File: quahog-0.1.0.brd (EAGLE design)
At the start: 71.3 x 17.9 mm, 33 parts, among them IC3 MCP1703CB, IC5 24AA128SN, J1 AYZ0202, X1 16 MHz

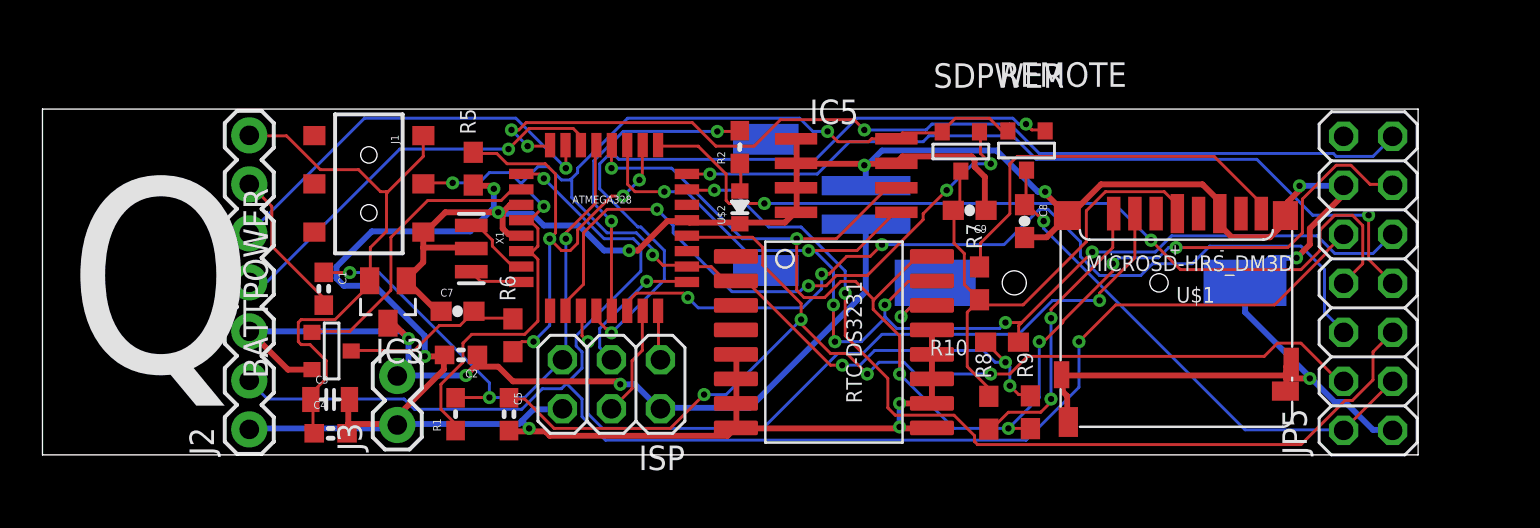
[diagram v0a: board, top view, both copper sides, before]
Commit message: update
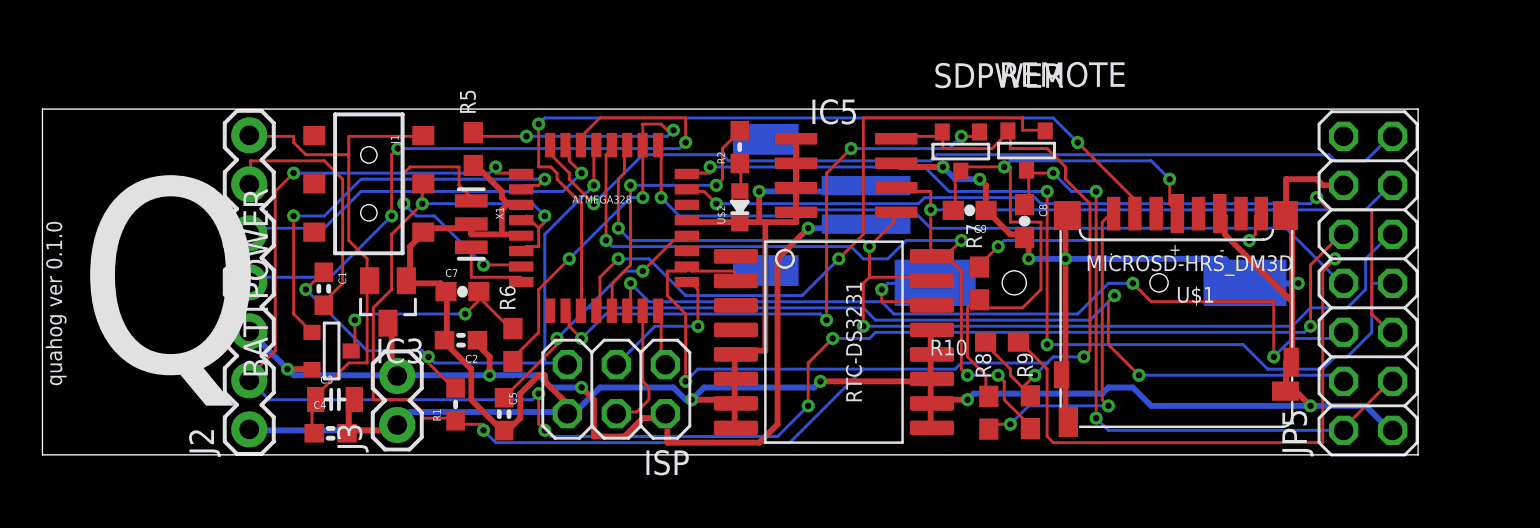
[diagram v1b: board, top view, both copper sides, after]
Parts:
- moved X1 1.27 mm to (22.2, 12.0)
- moved C7 1.05 mm to (21.8, 8.46)
- moved R5 1.02 mm to (22.3, 15.8)
- moved C2 0.76 mm to (21.7, 5.94)
- moved R1 0.51 mm to (21.4, 2.62)
- moved R6 0.51 mm to (24.4, 5.69)
- moved ISP 0.36 mm to (29.7, 3.40)
- moved C5 0.25 mm to (23.9, 2.11)
- moved C3 0.25 mm to (15.2, 2.87)
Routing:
- net SDA: track 60.8 -> 89.5 mm, vias 7 -> 4
- net VCC: track 86.2 -> 110.6 mm, vias 7 -> 6
- net D0_RX: track 21.1 -> 35.1 mm, vias 1 -> 3
- net N$1: track 3.66 -> 14.0 mm, vias 0 -> 2
- net D3: track 82.2 -> 90.6 mm, vias 2 -> 7
- net GND: track 201.4 -> 193.7 mm, vias 12 -> 10
- net N$7: track 27.1 -> 34.5 mm, vias 1 -> 3
- net A1: track 41.9 -> 49.2 mm, vias 2 -> 3
- net N$4: track 27.6 -> 33.9 mm, vias 0 -> 2
- net D4: track 15.5 -> 21.7 mm, vias 0 -> 2
- net N$20: track 7.88 -> 13.3 mm
- net A2: track 45.4 -> 40.3 mm, vias 2 -> 1
- net PWR: track 48.4 -> 53.5 mm, vias 3 -> 4
- net A0: track 48.3 -> 43.3 mm
- net N$16: track 20.7 -> 16.3 mm, vias 0 -> 2
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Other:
- board text added: "quahog ver 0.1.0"

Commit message: update
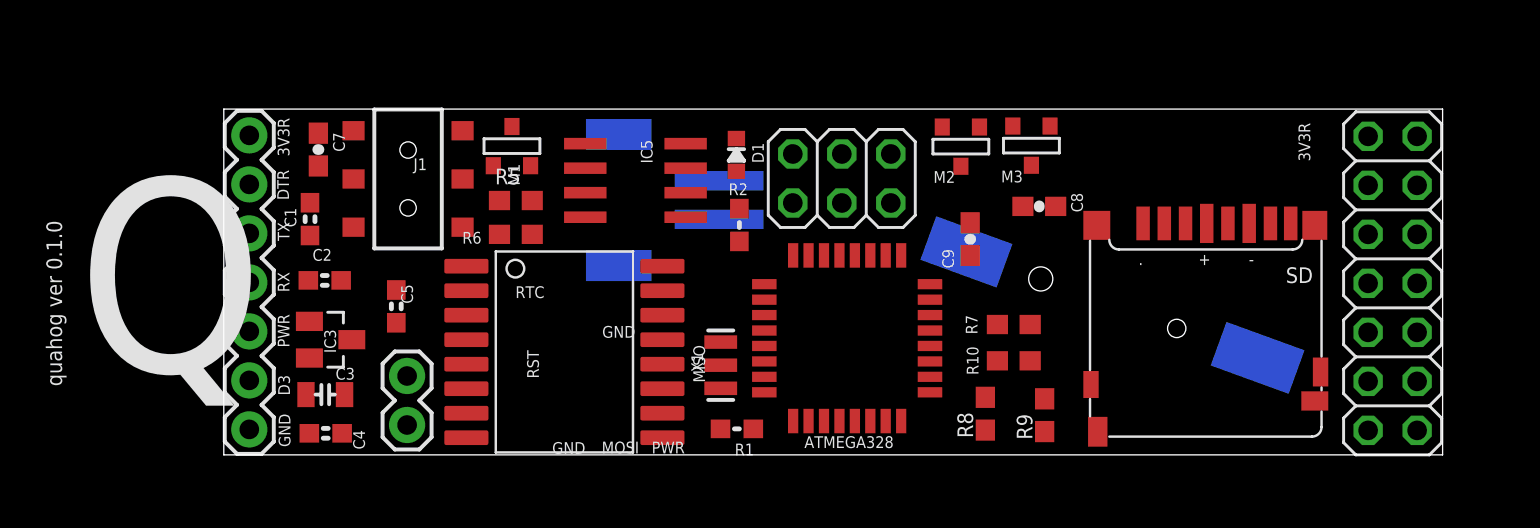
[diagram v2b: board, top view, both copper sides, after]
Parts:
- removed BATTPOWER, REMOTE, SDPWER: FDN340P, zetex:SOT-23
- removed RTC-DS3231: DS3231, _lh-library:DS3231
- removed U$1: MICROSD-HRS_DM3D, hrs_DM3D-SF:DM3D
- removed U$2: LED0603, LowPowerLab:0603-LED
- added D1: LED0603, LowPowerLab:0603-LED
- added M1, M2, M3: FDN340P, zetex:SOT-23
- added RTC: DS3231, _lh-library:DS3231
- added SD: MICROSD-HRS_DM3D, hrs_DM3D-SF:DM3D
- moved ISP 16.0 mm to (41.4, 14.3)
- moved X1 14.9 mm to (35.2, 4.65)
- moved R1 14.6 mm to (36.0, 1.35), turned to 180 degrees
- moved ATMEGA328 13.8 mm to (41.7, 6.05), turned to 180 degrees
- moved IC5 10.9 mm to (30.7, 14.2), turned to 90 degrees
- moved C7 10.5 mm to (14.3, 15.8), turned to 270 degrees
- moved C5 7.90 mm to (18.3, 7.70)
- moved C2 7.71 mm to (14.6, 9.04), turned to 0 degrees
- moved CN2 7.62 mm to (31.4, 13.2)
- moved R6 5.74 mm to (24.5, 11.4), turned to 180 degrees
- moved R2 4.04 mm to (36.1, 11.9), turned to 270 degrees
- moved C1 3.68 mm to (13.9, 12.2), turned to 90 degrees
- moved IC3 3.56 mm to (14.9, 5.97), turned to 270 degrees
- moved R5 3.46 mm to (24.5, 13.2), turned to 180 degrees
- moved R7 2.78 mm to (50.3, 6.76), turned to 180 degrees
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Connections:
- removed net D11_MOSI: ATMEGA328.15, ISP.4
- removed net D12_MISO: ATMEGA328.16, ISP.1
- removed net D13_SCK: ATMEGA328.17, ISP.3
- removed net D5/RTC: RTC-DS3231.3
- removed net VBAT: JP5.14
- net A2: now also JP5.10; no longer JP5.8
- net A3: now also JP5.8
- net AREF: now also JP5.2; no longer JP5.4
- net D10: now also JP5.4; no longer JP5.6
- net D3: now also JP5.6; no longer JP5.10
- net D4: now also M1.3; no longer BATTPOWER.3
- net D5: now also RTC.3
- net D6: now also M2.3; no longer SDPWER.3
- net D7: now also SD.CD/DAT3; no longer U$1.CD/DAT3
- net D8: now also M3.3; no longer REMOTE.3
- net GND: now also D1.MINUS, RTC.10, RTC.11, RTC.12, RTC.13, RTC.5, RTC.6, RTC.7, RTC.8, RTC.9, SD.GND1, SD.GND2, SD.GND3, SD.GND4, SD.SW_A, SD.SW_B, SD.VSS; no longer RTC-DS3231.10, RTC-DS3231.11, RTC-DS3231.12, RTC-DS3231.13, RTC-DS3231.5, RTC-DS3231.6, RTC-DS3231.7, RTC-DS3231.8, RTC-DS3231.9, U$1.GND1, U$1.GND2, U$1.GND3, U$1.GND4, U$1.SW_A, U$1.SW_B, U$1.VSS, U$2.MINUS
- net MISO: now also ATMEGA328.16, ISP.1, SD.DAT0; no longer U$1.DAT0
- net MOSI: now also ATMEGA328.15, ISP.4, SD.CMD; no longer U$1.CMD
- net N$15: now also M1.1; no longer BATTPOWER.1
- net N$16: now also SD.DAT1; no longer U$1.DAT1
- net N$18: now also SD.DAT2; no longer U$1.DAT2
- net N$2: now also D1.PLUS; no longer U$2.PLUS
- net N$4: now also M2.1, SD.VDD; no longer SDPWER.1, U$1.VDD
- net N$7: now also M3.1; no longer JP5.2, REMOTE.1
- net PWR: now also JP5.14, M1.2; no longer BATTPOWER.2
- net RTC_BATT: now also RTC.14; no longer RTC-DS3231.14
- net SCK: now also ATMEGA328.17, ISP.3, SD.CLK; no longer U$1.CLK
- net SCL: now also RTC.16; no longer RTC-DS3231.16
- net SDA: now also RTC.15; no longer RTC-DS3231.15
- net VCC: now also M2.2, M3.2, RTC.2; no longer REMOTE.2, RTC-DS3231.2, SDPWER.2
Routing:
- net GND: track 193.7 -> 0.00 mm, vias 10 -> 0
- net VCC: track 110.6 -> 0.00 mm, vias 6 -> 0
- net D3: track 90.6 -> 0.00 mm, vias 7 -> 0
- net SDA: track 89.5 -> 0.00 mm, vias 4 -> 0
- net SCL: track 68.5 -> 0.00 mm, vias 5 -> 0
- net AREF: track 57.0 -> 0.00 mm, vias 4 -> 0
- net PWR: track 53.5 -> 0.00 mm, vias 4 -> 0
- net A1: track 49.2 -> 0.00 mm, vias 3 -> 0
- net D2: track 47.3 -> 0.00 mm, vias 1 -> 0
- net D7: track 44.5 -> 0.00 mm, vias 2 -> 0
- net D10: track 43.5 -> 0.00 mm, vias 3 -> 0
- net A0: track 43.3 -> 0.00 mm, vias 2 -> 0
- net A2: track 40.3 -> 0.00 mm, vias 1 -> 0
- net D0_RX: track 35.1 -> 0.00 mm, vias 3 -> 0
- net N$7: track 34.5 -> 0.00 mm, vias 3 -> 0
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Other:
- board size 71.3 x 17.9 mm -> 63.2 x 17.9 mm
- board text added: "3V3R"
- board text added: "D3"
- board text added: "DTR"
- board text added: "GND"
- board text added: "MISO"
- board text added: "MOSI"
- board text added: "PWR"
- board text added: "RST"
- board text added: "RX"
- board text added: "TX"

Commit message: update
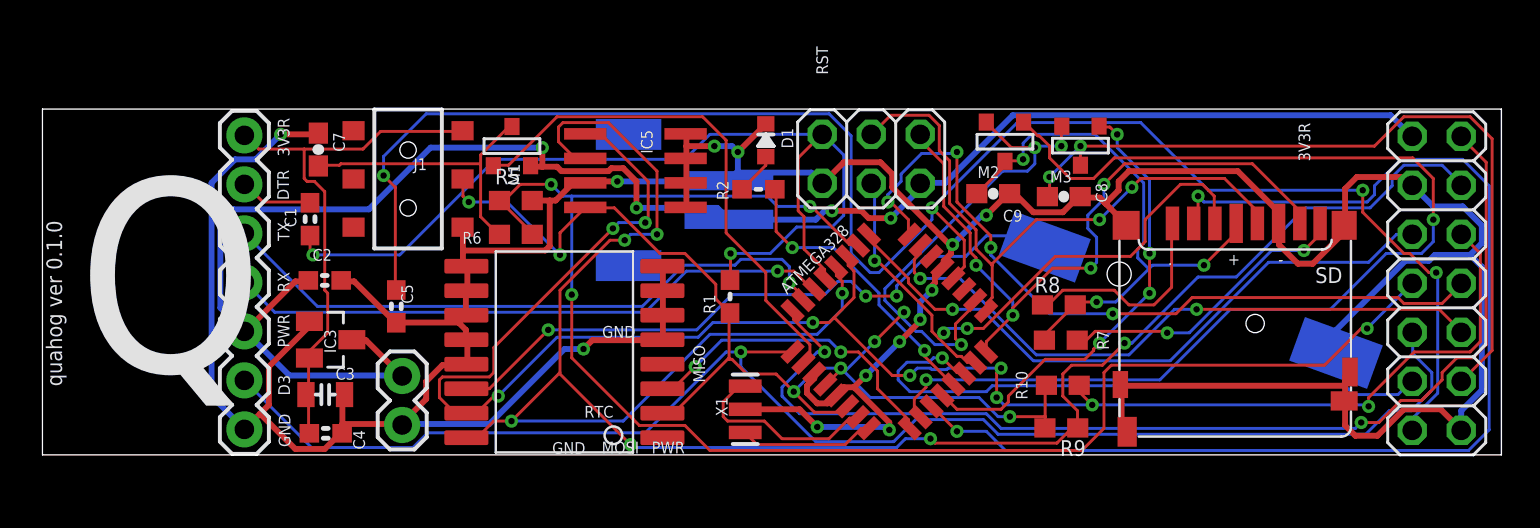
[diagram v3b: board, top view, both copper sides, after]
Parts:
- moved R1 6.87 mm to (35.6, 8.20), turned to 90 degrees
- moved R8 6.81 mm to (52.7, 7.77), turned to 0 degrees
- moved BAT 4.07 mm to (55.8, 9.37)
- moved R10 2.84 mm to (52.9, 3.61)
- moved C9 2.65 mm to (49.3, 13.5), turned to 180 degrees
- moved X1 2.62 mm to (36.4, 2.36)
- moved R7 2.57 mm to (52.8, 5.94), turned to 0 degrees
- moved M3 2.54 mm to (53.8, 16.0)
- moved M2 2.30 mm to (49.9, 16.2)
- moved JP5 2.29 mm to (72.3, 8.89)
- moved ATMEGA328 2.21 mm to (43.9, 6.40), turned to 45 degrees
- moved R2 2.10 mm to (37.1, 13.8), turned to 0 degrees
- moved ISP 1.83 mm to (43.0, 15.3)
- moved D1 1.70 mm to (37.5, 16.3)
- moved SD 1.52 mm to (67.8, 12.4)
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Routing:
- net GND: track 0.00 -> 229.3 mm, vias 0 -> 13
- net SCL: track 0.00 -> 108.7 mm, vias 0 -> 7
- net SDA: track 0.00 -> 94.7 mm, vias 0 -> 9
- net PWR: track 0.00 -> 93.3 mm, vias 0 -> 4
- net AREF: track 0.00 -> 90.4 mm, vias 0 -> 4
- net VCC: track 0.00 -> 82.9 mm, vias 0 -> 10
- net A3: track 0.00 -> 82.1 mm, vias 0 -> 4
- net D3: track 0.00 -> 75.2 mm, vias 0 -> 1
- net D7: track 0.00 -> 61.4 mm, vias 0 -> 2
- net D6: track 0.00 -> 58.5 mm, vias 0 -> 2
- net D2: track 0.00 -> 56.8 mm, vias 0 -> 2
- net RST: track 0.00 -> 51.4 mm, vias 0 -> 2
- net A1: track 0.00 -> 40.0 mm, vias 0 -> 4
- net N$7: track 0.00 -> 40.0 mm, vias 0 -> 2
- net MISO: track 0.00 -> 36.3 mm, vias 0 -> 4
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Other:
- board size 63.2 x 17.9 mm -> 75.6 x 17.9 mm
